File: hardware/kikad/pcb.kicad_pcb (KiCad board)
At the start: 2 copper layers, 45 x 45 mm, 22 parts, among them J1 LED, J2 BOARD

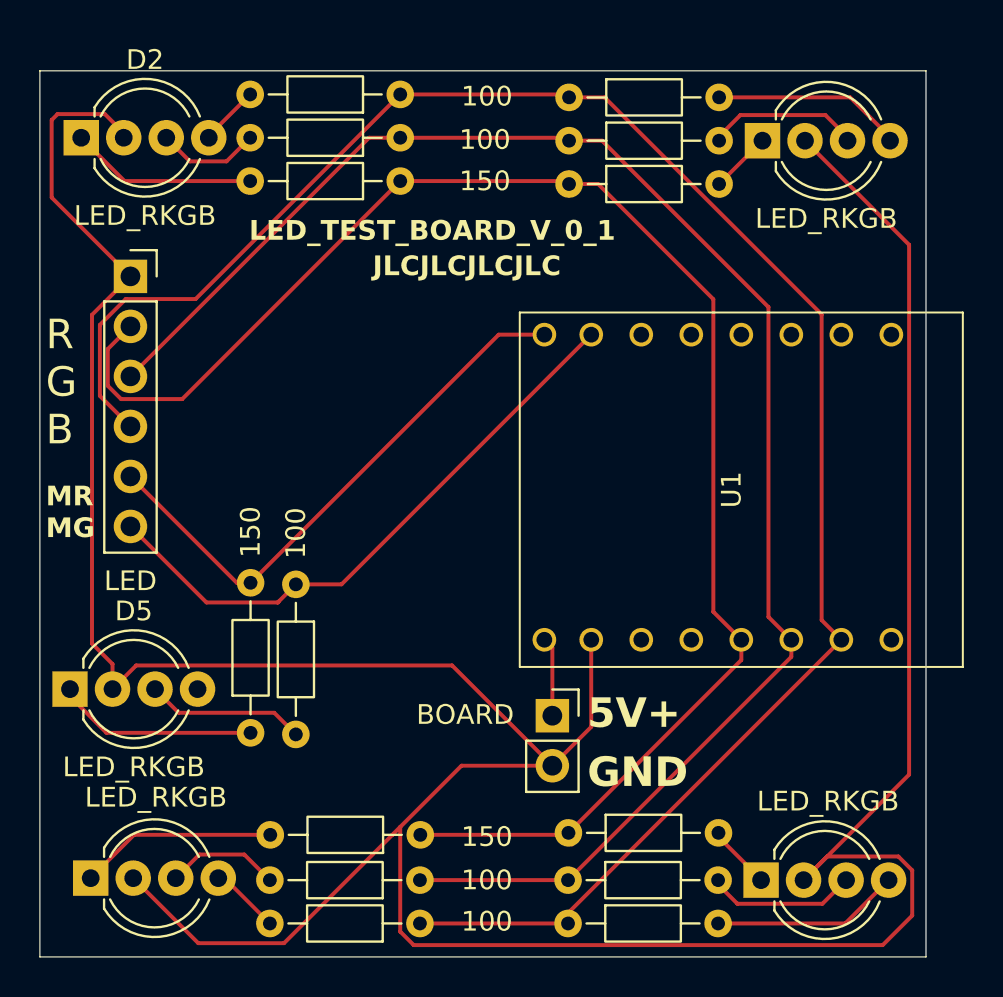
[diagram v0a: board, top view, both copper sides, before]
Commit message: organization
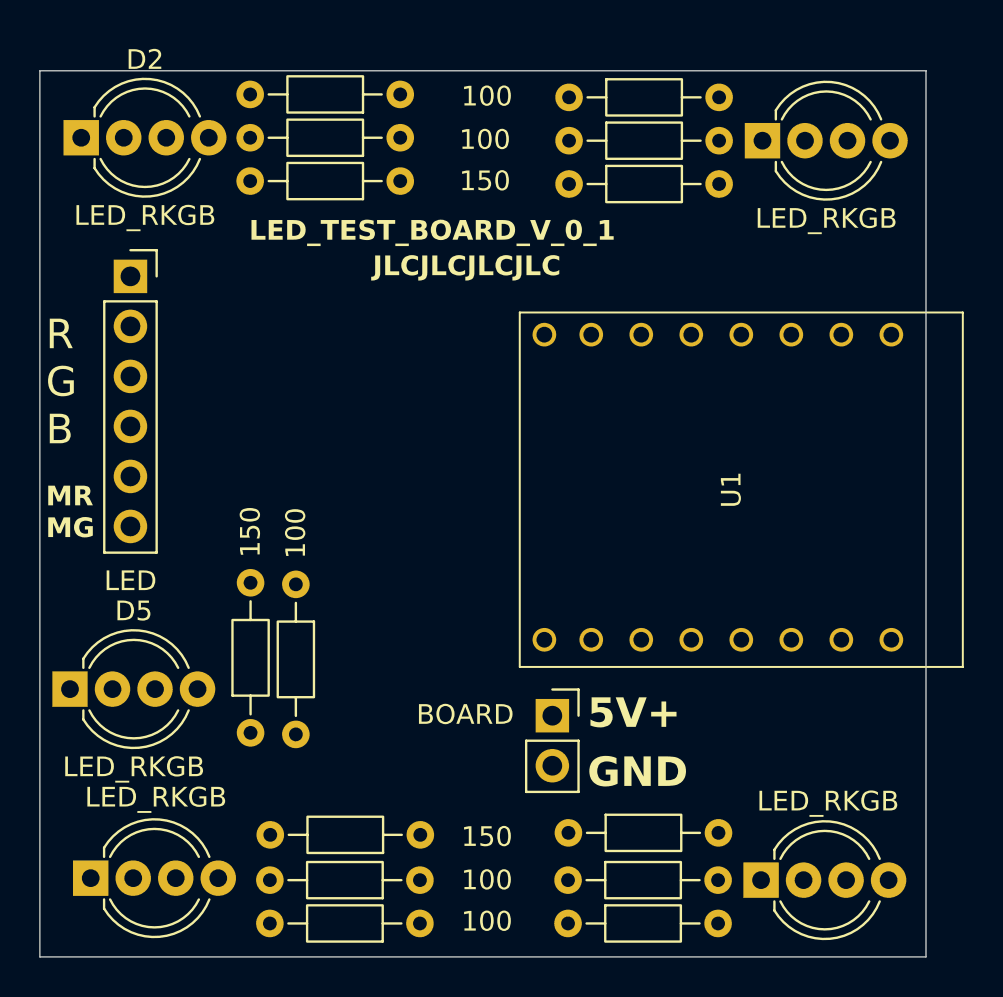
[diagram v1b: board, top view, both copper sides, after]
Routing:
- net GND: track 177.9 -> 0.00 mm
- net /B: track 98.1 -> 0.00 mm
- net /G: track 83.9 -> 0.00 mm
- net /R: track 81.1 -> 0.00 mm
- net Net-(J1-Pin_6): track 30.7 -> 0.00 mm
- net Net-(J1-Pin_5): track 28.5 -> 0.00 mm
- net Net-(D5-RA): track 11.0 -> 0.00 mm
- net Net-(D4-RA): track 10.9 -> 0.00 mm
- net Net-(D1-BA): track 9.63 -> 0.00 mm
- net Net-(D3-BA): track 9.57 -> 0.00 mm
- net Net-(D2-RA): track 9.49 -> 0.00 mm
- net Net-(D5-GA): track 8.10 -> 0.00 mm
- net Net-(D1-GA): track 7.76 -> 0.00 mm
- net Net-(D3-GA): track 7.62 -> 0.00 mm
- net Net-(D4-GA): track 5.82 -> 0.00 mm
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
